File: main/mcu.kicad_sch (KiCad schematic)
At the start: 13 parts, among them J501 Conn_ARM_JTAG_SWD_20, SW501 B3SL-1022P, U501 STM32L476RGTx, Y501 8MHz

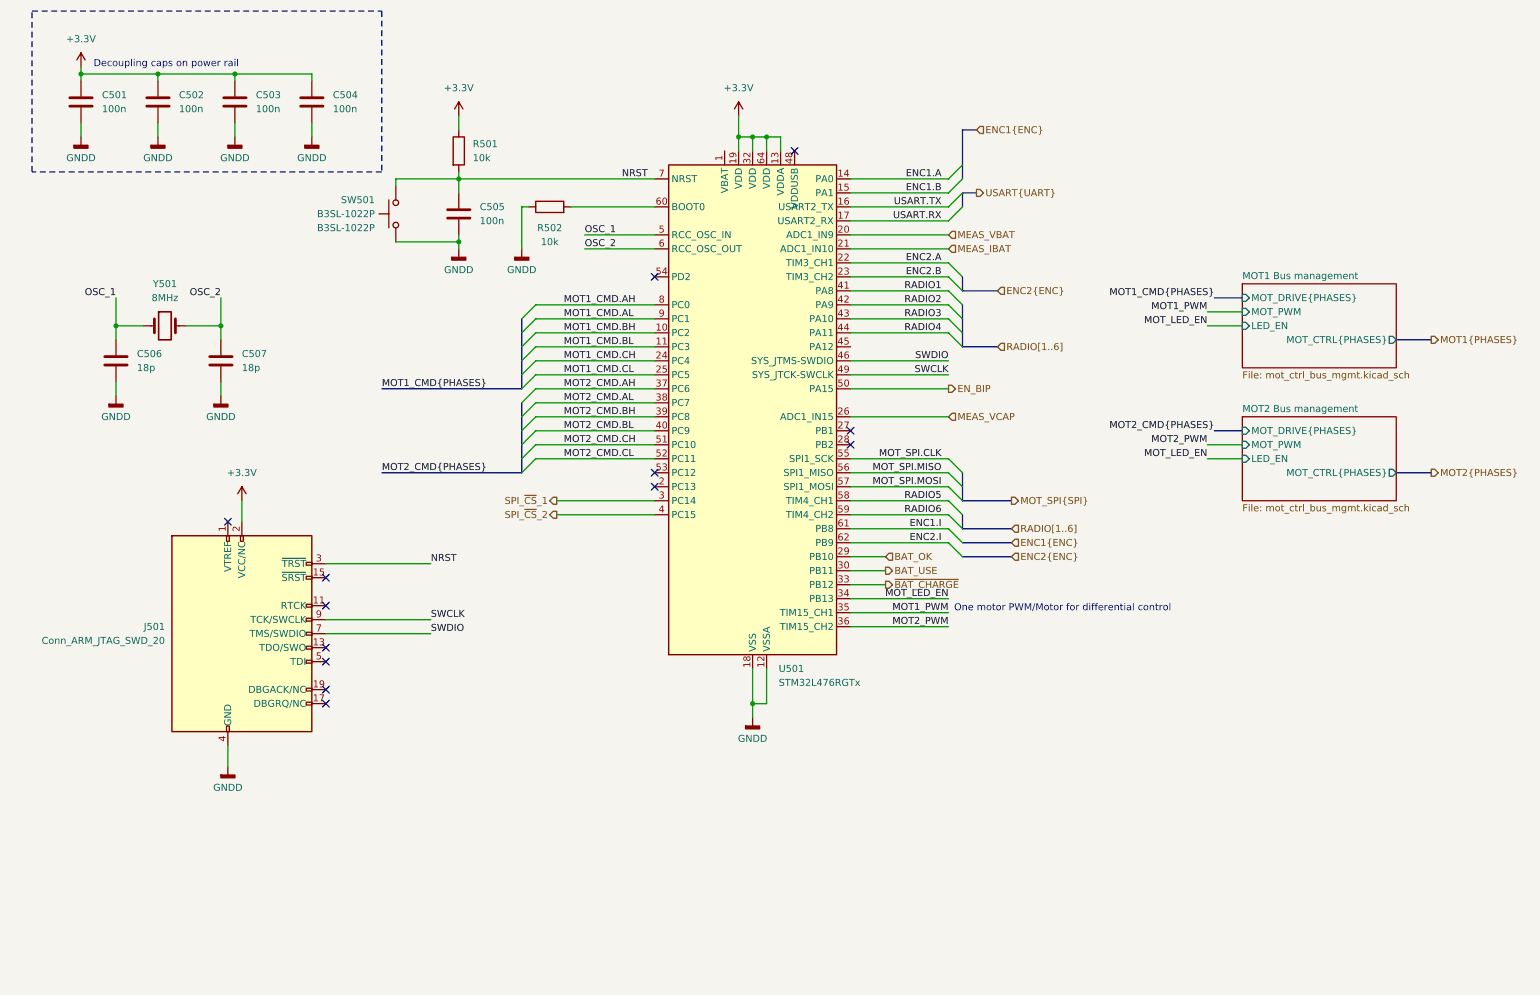
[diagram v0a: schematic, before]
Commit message: Tapeout
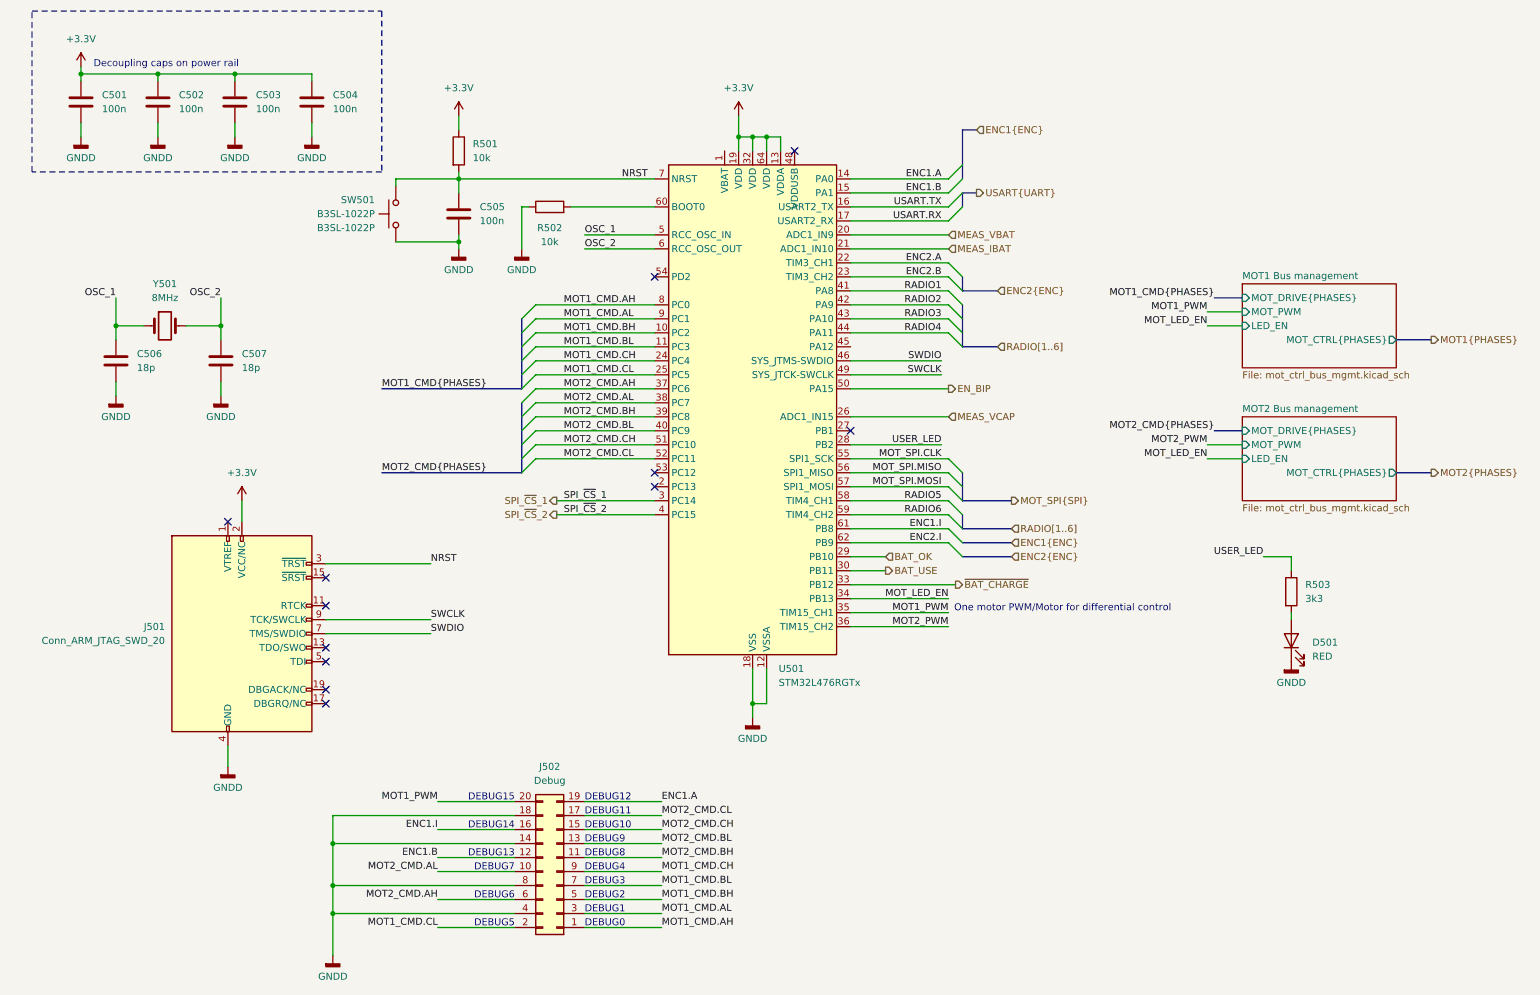
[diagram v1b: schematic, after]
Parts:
- added D501: RED, LED_SMD:LED_0805_2012Metric, symbol Device:LED
- added J502: Debug, Connector_IDC:IDC-Header_2x10_P2.54mm_Vertical, symbol Connector_Generic:Conn_02x10_Odd_Even
- added R503: 3k3, Resistor_SMD:R_0805_2012Metric, symbol Device:R
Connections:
- net ENC1.A: now also J502.19 (Pin_19)
- net ENC1.B: now also J502.12 (Pin_12)
- net ENC1.I: now also J502.16 (Pin_16)
- net GNDD: now also D501.1 (K), J502.14 (Pin_14), J502.18 (Pin_18), J502.4 (Pin_4), J502.8 (Pin_8)
- net MOT1_CMD.AH: now also J502.1 (Pin_1)
- net MOT1_CMD.AL: now also J502.3 (Pin_3)
- net MOT1_CMD.BH: now also J502.5 (Pin_5)
- net MOT1_CMD.BL: now also J502.7 (Pin_7)
- net MOT1_CMD.CH: now also J502.9 (Pin_9)
- net MOT1_CMD.CL: now also J502.2 (Pin_2)
- net MOT1_PWM: now also J502.20 (Pin_20)
- net MOT2_CMD.AH: now also J502.6 (Pin_6)
- net MOT2_CMD.AL: now also J502.10 (Pin_10)
- net MOT2_CMD.BH: now also J502.11 (Pin_11)
- net MOT2_CMD.BL: now also J502.13 (Pin_13)
- net MOT2_CMD.CH: now also J502.15 (Pin_15)
- net MOT2_CMD.CL: now also J502.17 (Pin_17)
- net USER_LED: now reaches U501.28 (PB2)
- net USER_LED: now also R503.1
- new net: D501.2 (A), R503.2
- no-connect marks 13 -> 12
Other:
- note added: "DEBUG0"
- note added: "DEBUG1"
- note added: "DEBUG10"
- note added: "DEBUG11"
- note added: "DEBUG12"
- note added: "DEBUG13"
- note added: "DEBUG14"
- note added: "DEBUG15"
- note added: "DEBUG2"
- note added: "DEBUG3"
- note added: "DEBUG4"
- note added: "DEBUG5"
- note added: "DEBUG6"
- note added: "DEBUG7"
- note added: "DEBUG8"
- note added: "DEBUG9"

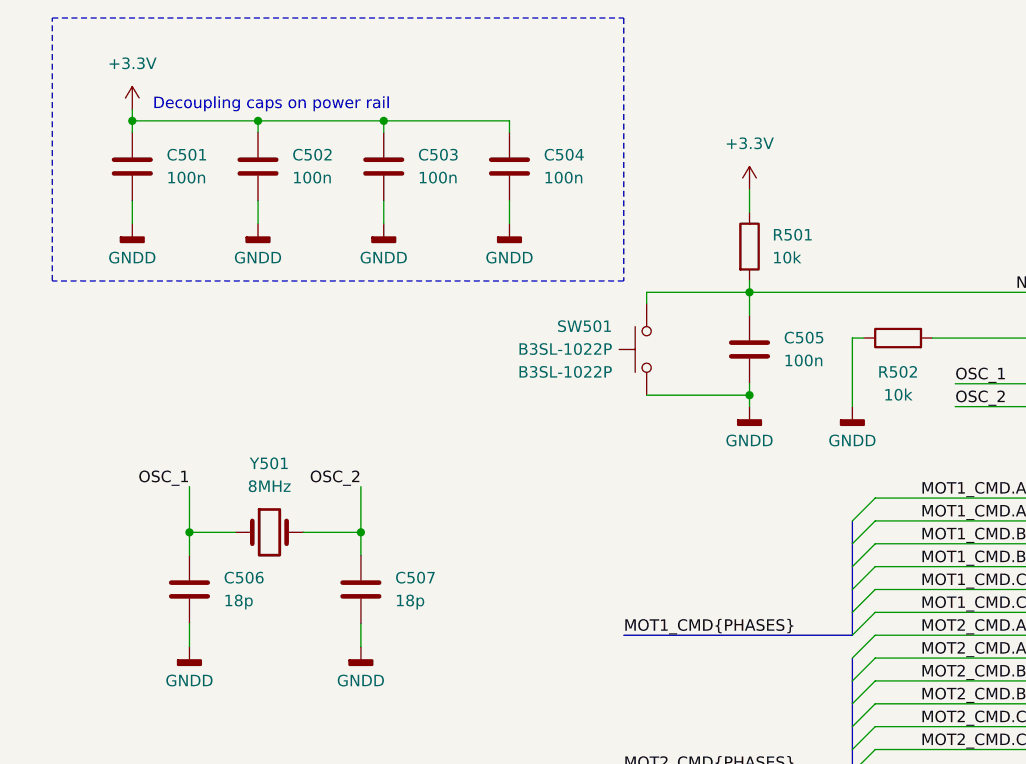
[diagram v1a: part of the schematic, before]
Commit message: Sent to fab
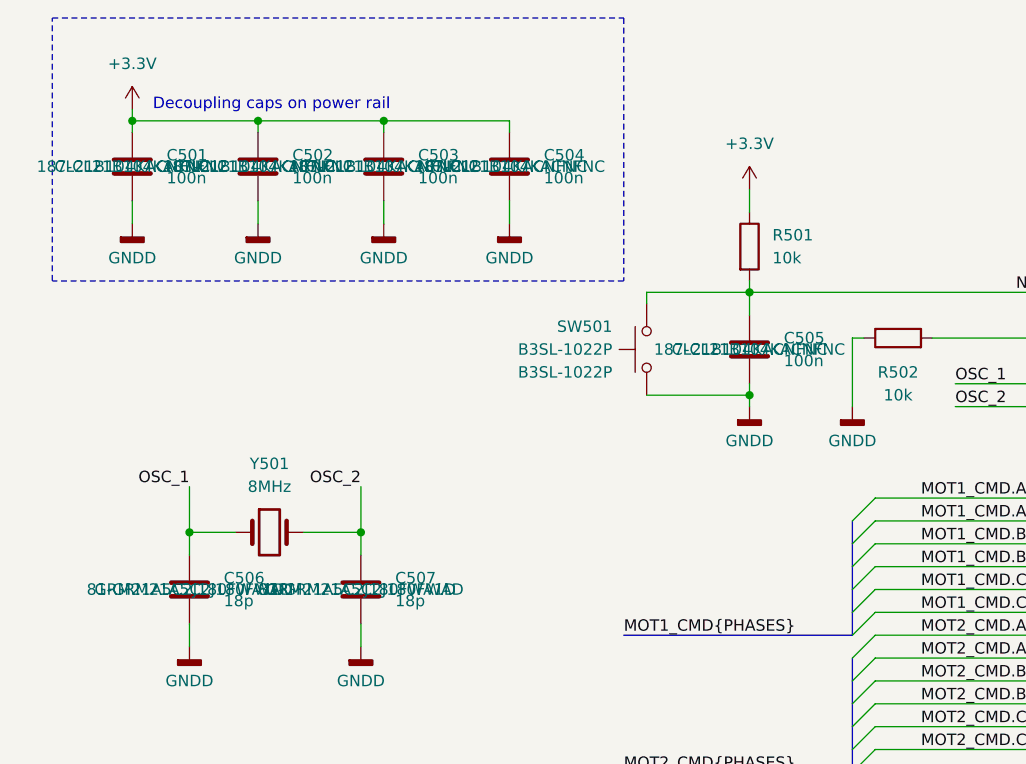
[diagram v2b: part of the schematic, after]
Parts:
- C501, C502, C503, C504, C505: MPN (none) -> CL21B104KACNFNC; Mouser SKU (none) -> 187-CL21B104KACNFNC
- C506, C507: MPN (none) -> GRM21A5C2J180FWA1D; Mouser SKU (none) -> 81-GRM21A5C2J180FWAD
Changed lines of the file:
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@@
+			)
+		)
+		(property "Quantity" ""
+			(at 78.74 49.53 0)
+			(effects
+				(font
+					(size 1.27 1.27)
+				)
 			)
 		)
@@
 			)
 		)
+		(property "MPN" "CL21B104KACNFNC "
+			(at 63.5 29.21 0)
+			(effects
+				(font
+					(size 1.27 1.27)
+				)
+			)
+		)
+		(property "Mouser SKU" " 187-CL21B104KACNFNC "
+			(at 63.5 29.21 0)
+			(effects
+				(font
+					(size 1.27 1.27)
+				)
+			)
+		)
+		(property "Quantity" ""
+			(at 63.5 29.21 0)
+			(effects
+				(font
+					(size 1.27 1.27)
+				)
+			)
+		)
 		(pin "1"
 		)
@@
 				)
 				(hide yes)
+			)
+		)
+		(property "Quantity" ""
+			(at 241.3 118.11 0)
+			(effects
+				(font
+					(size 1.27 1.27)
+				)
 			)
 		)
@@
 			)
 		)
+		(property "MPN" "GRM21A5C2J180FWA1D"
+			(at 46.99 76.2 0)
+			(effects
+				(font
+					(size 1.27 1.27)
+				)
+			)
+		)
+		(property "Mouser SKU" " 81-GRM21A5C2J180FWAD "
+			(at 46.99 76.2 0)
+			(effects
+				(font
+					(size 1.27 1.27)
+				)
+			)
+		)
+		(property "Quantity" ""
+			(at 46.99 76.2 0)
+			(effects
+				(font
+					(size 1.27 1.27)
+				)
+			)
+		)
 		(pin "1"
 		)
@@
 			)
 		)
+		(property "Quantity" ""
+			(at 50.8 125.73 0)
+			(effects
+				(font
+					(size 1.27 1.27)
+				)
+			)
+		)
 		(pin "8"
 		)
@@
 			)
 		)
+		(property "MPN" "GRM21A5C2J180FWA1D"
+			(at 27.94 76.2 0)
+			(effects
+				(font
+					(size 1.27 1.27)
+				)
+			)
+		)
+		(property "Mouser SKU" " 81-GRM21A5C2J180FWAD "
+			(at 27.94 76.2 0)
+			(effects
+				(font
+					(size 1.27 1.27)
+				)
+			)
+		)
+		(property "Quantity" ""
+			(at 27.94 76.2 0)
+			(effects
+				(font
+					(size 1.27 1.27)
+				)
+			)
+		)
 		(pin "1"
 		)
@@
 			)
 		)
+		(property "Quantity" ""
+			(at 106.68 48.26 0)
+			(effects
+				(font
+					(size 1.27 1.27)
+				)
+			)
+		)
 		(pin "2"
 		)
@@
 			)
 		)
+		(property "Quantity" ""
+			(at 107.95 168.91 0)
+			(effects
+				(font
+					(size 1.27 1.27)
+				)
+			)
+		)
 		(pin "13"
 		)
@@
 			)
 		)
+		(property "Quantity" ""
+			(at 90.17 38.1 0)
+			(effects
+				(font
+					(size 1.27 1.27)
+				)
+			)
+		)
 		(pin "2"
 		)
@@
 			)
 		)
+		(property "MPN" "CL21B104KACNFNC "
+			(at 35.56 29.21 0)
+			(effects
+				(font
+					(size 1.27 1.27)
+				)
+			)
+		)
+		(property "Mouser SKU" " 187-CL21B104KACNFNC "
+			(at 35.56 29.21 0)
+			(effects
+				(font
+					(size 1.27 1.27)
+				)
+			)
+		)
+		(property "Quantity" ""
+			(at 35.56 29.21 0)
+			(effects
+				(font
+					(size 1.27 1.27)
+				)
+			)
+		)
 		(pin "1"
 		)
@@
 			)
 		)
+		(property "Quantity" ""
+			(at 36.83 69.85 0)
+			(effects
+				(font
+					(size 1.27 1.27)
+				)
+			)
+		)
 		(pin "1"
 		)
@@
 			)
 		)
+		(property "MPN" "CL21B104KACNFNC "
+			(at 90.17 49.53 0)
+			(effects
+				(font
+					(size 1.27 1.27)
+				)
+			)
+		)
+		(property "Mouser SKU" " 187-CL21B104KACNFNC "
+			(at 90.17 49.53 0)
+			(effects
+				(font
+					(size 1.27 1.27)
+				)
+			)
+		)
+		(property "Quantity" ""
+			(at 90.17 49.53 0)
+			(effects
+				(font
+					(size 1.27 1.27)
+				)
+			)
+		)
 		(pin "1"
 		)
@@
 			)
 		)
+		(property "Quantity" ""
+			(at 143.51 86.36 0)
+			(effects
+				(font
+					(size 1.27 1.27)
+				)
+			)
+		)
 		(pin "30"
 		)
@@
 			)
 		)
+		(property "MPN" "CL21B104KACNFNC "
+			(at 49.53 29.21 0)
+			(effects
+				(font
+					(size 1.27 1.27)
+				)
+			)
+		)
+		(property "Mouser SKU" " 187-CL21B104KACNFNC "
+			(at 49.53 29.21 0)
+			(effects
+				(font
+					(size 1.27 1.27)
+				)
+			)
+		)
+		(property "Quantity" ""
+			(at 49.53 29.21 0)
+			(effects
+				(font
+					(size 1.27 1.27)
+				)
+			)
+		)
 		(pin "1"
 		)
@@
 			)
 		)
+		(property "Quantity" ""
+			(at 241.3 127 0)
+			(effects
+				(font
+					(size 1.27 1.27)
+				)
+			)
+		)
 		(pin "1"
 		)
@@
 			)
 		)
+		(property "MPN" "CL21B104KACNFNC "
+			(at 21.59 29.21 0)
+			(effects
+				(font
+					(size 1.27 1.27)
+				)
+			)
+		)
+		(property "Mouser SKU" " 187-CL21B104KACNFNC "
+			(at 21.59 29.21 0)
+			(effects
+				(font
+					(size 1.27 1.27)
+				)
+			)
+		)
+		(property "Quantity" ""
+			(at 21.59 29.21 0)
+			(effects
+				(font
+					(size 1.27 1.27)
+				)
+			)
+		)
